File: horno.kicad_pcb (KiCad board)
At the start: 2 copper layers, 96.2 x 116 mm, 25 parts, among them T1 25, U1 AD596AHZ, U2 STM32F103C8Tx, U3 LM78M05_TO220, U4 LM78M05_TO220

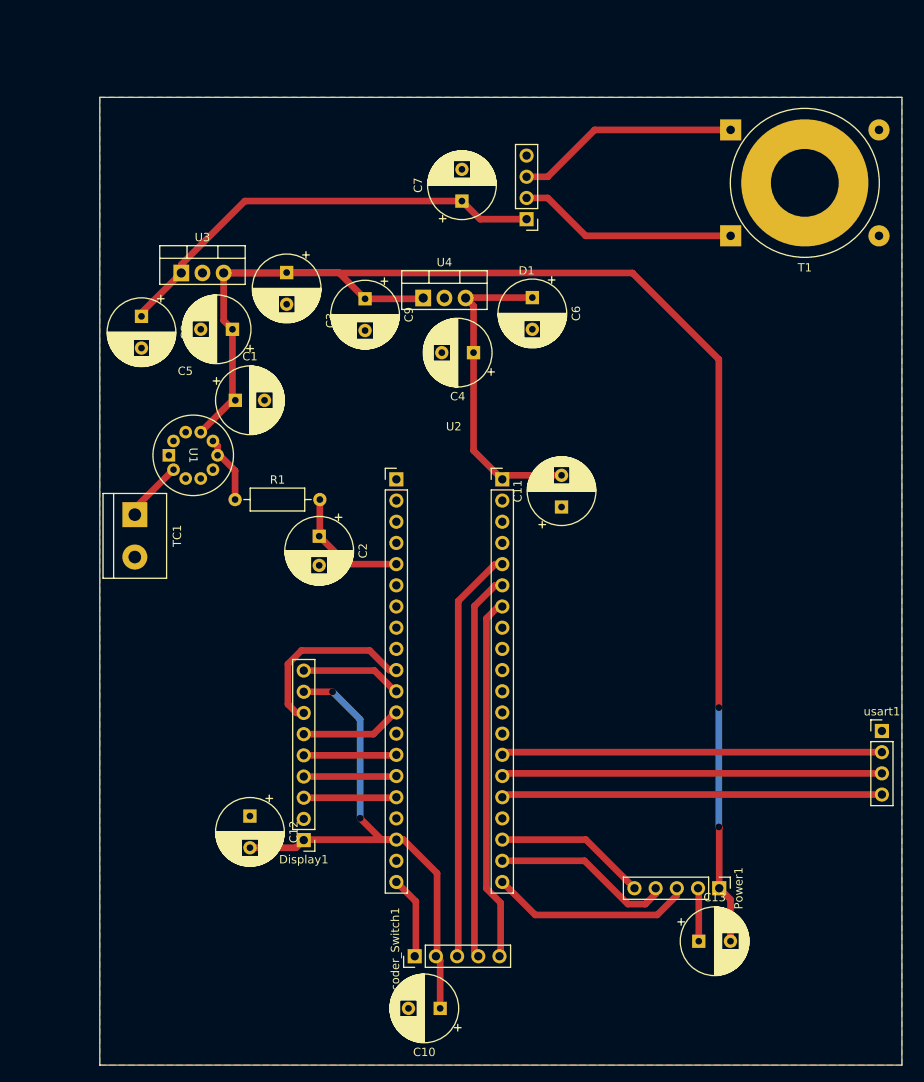
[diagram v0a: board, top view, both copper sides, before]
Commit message: com
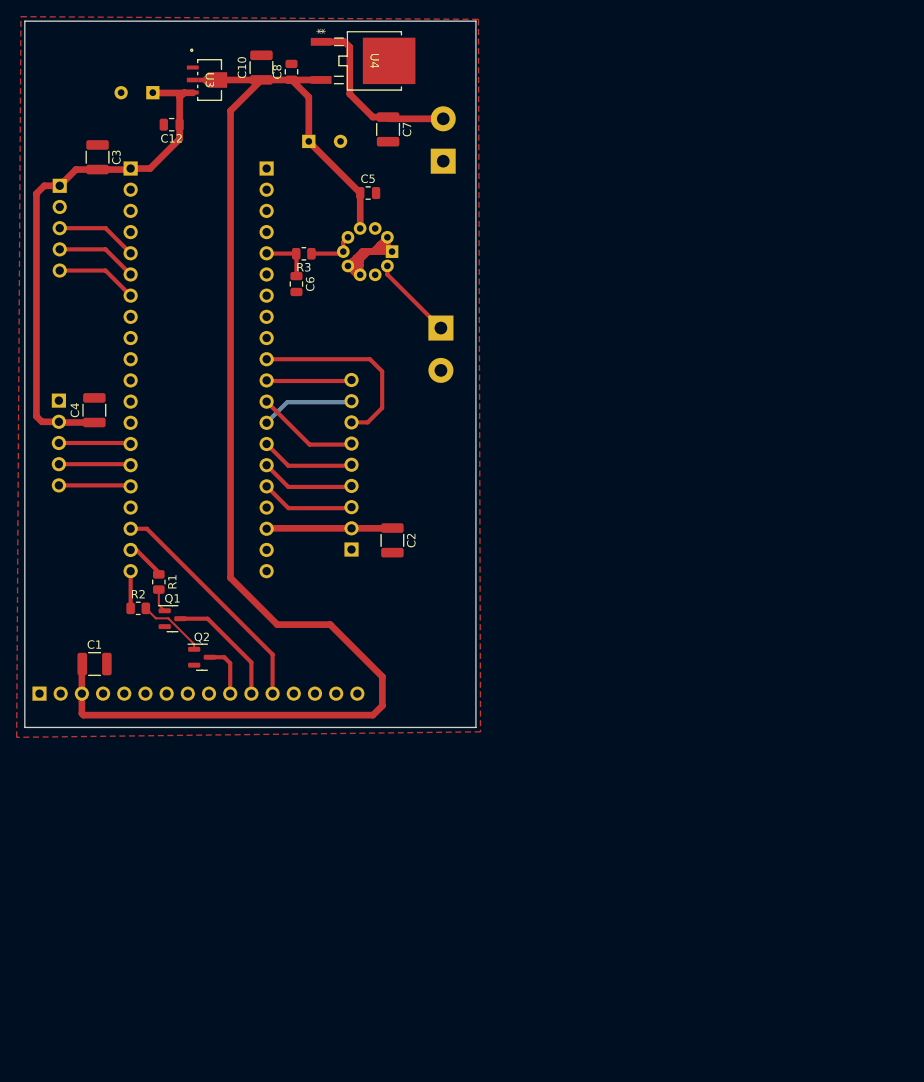
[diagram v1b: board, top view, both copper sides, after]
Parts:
- removed C13: 100n, Capacitor_THT:CP_Radial_D8.0mm_P3.80mm
- removed D1: D_Bridge_+-AA, Connector_PinHeader_2.54mm:PinHeader_1x04_P2.54mm_Vertical
- removed Power1: Conn_01x05_Pin, Connector_PinHeader_2.54mm:PinHeader_1x05_P2.54mm_Vertical
- removed T1: 25, Transformer_THT:Transformer_Toroid_Horizontal_D18.0mm
- removed usart1: Conn_01x04_Pin, Connector_PinHeader_2.54mm:PinHeader_1x04_P2.54mm_Vertical
- added PWR1: Conn_01x16_Pin, Connector_PinHeader_2.54mm:PinHeader_1x16_P2.54mm_Horizontal, B.Cu at (37.5, 178.8)
- added Q1: BC848, Package_TO_SOT_SMD:SOT-23, F.Cu at (53.5, 169.8)
- added Q2: BC848, Package_TO_SOT_SMD:SOT-23, F.Cu at (57.0, 174.5)
- added R2: 4.7k, Resistor_SMD:R_0805_2012Metric, F.Cu at (49.4, 168.6)
- added R3: 33k, Resistor_SMD:R_0805_2012Metric, F.Cu at (69.2, 126.1)
- added USART1: Conn_01x05_Pin, Connector_PinHeader_2.54mm:PinHeader_1x05_P2.54mm_Vertical, B.Cu at (39.9, 143.7)
- added Vin1: Conn_01x02, TerminalBlock:TerminalBlock_bornier-2_P5.08mm, B.Cu at (85.9, 115.0)
- C1: value 0.01u -> 100n; footprint Capacitor_THT:CP_Radial_D8.0mm_P3.50mm -> Capacitor_SMD:C_1210_3225Metric
- C10: footprint Capacitor_THT:CP_Radial_D8.0mm_P3.80mm -> Capacitor_SMD:C_1210_3225Metric
- C11, C9: value 100n -> 47u; moved to B.Cu
- C12, C8: value 100n -> 0.1u; footprint Capacitor_THT:CP_Radial_D8.0mm_P3.80mm -> Capacitor_SMD:C_0805_2012Metric
- C2: value 470n -> 100n; footprint Capacitor_THT:CP_Radial_D8.0mm_P3.50mm -> Capacitor_SMD:C_1210_3225Metric
- C3, C4: value 47u -> 100n; footprint Capacitor_THT:CP_Radial_D8.0mm_P3.80mm -> Capacitor_SMD:C_1210_3225Metric
- C5: value 0.1u -> 0.01u; footprint Capacitor_THT:CP_Radial_D8.0mm_P3.80mm -> Capacitor_SMD:C_0805_2012Metric
- C6: value 0.1u -> 470n; footprint Capacitor_THT:CP_Radial_D8.0mm_P3.80mm -> Capacitor_SMD:C_0805_2012Metric
- C7: value 470u -> 100n; footprint Capacitor_THT:CP_Radial_D8.0mm_P3.80mm -> Capacitor_SMD:C_1210_3225Metric
- Display1, Encoder_Switch1, TC1: moved to B.Cu
- R1: value 33k -> 4.7k; footprint Resistor_THT:R_Axial_DIN0207_L6.3mm_D2.5mm_P10.16mm_Horizontal -> Resistor_SMD:R_0805_2012Metric
- U1: value AD596AHZ -> STM32F103C8Tx; footprint ad596:ad596 -> blue_pill:blue_pill; moved to B.Cu
- U2: value STM32F103C8Tx -> AD596AHZ; footprint blue_pill:blue_pill -> ad596:ad596; moved to B.Cu
- U3: value LM78M05_TO220 -> MCP1700T-3302E/MB; footprint Package_TO_SOT_THT:TO-220-3_Vertical -> reg33:SOT-89_3MC_MCH
- U4: value LM78M05_TO220 -> L78M05CDT-TR; footprint Package_TO_SOT_THT:TO-220-3_Vertical -> reg5:DPAK_STM
- moved C10 114.8 mm to (64.1, 103.8), turned to 90 degrees
- moved Encoder_Switch1 101.7 mm to (40.0, 118.0), turned to 180 degrees
- moved C12 83.4 mm to (53.4, 110.6), turned to 180 degrees
- moved C11 53.3 mm to (69.8, 112.6), turned to 0 degrees
- moved C4 46.0 mm to (44.1, 144.8), turned to 90 degrees
- moved TC1 43.0 mm to (85.6, 135.0)
- moved U1 40.5 mm to (57.9, 110.0), turned to 180 degrees
- moved C1 35.8 mm to (44.1, 175.3)
- moved C9 35.5 mm to (51.1, 106.8), turned to 180 degrees
- moved Display1 35.3 mm to (74.9, 161.6), turned to 0 degrees
- moved C8 34.4 mm to (67.7, 104.3), turned to 90 degrees
- moved U4 29.0 mm to (77.7, 103.0), turned to -90 degrees
- moved C6 28.3 mm to (68.3, 129.7)
- moved C3 26.6 mm to (44.5, 114.5)
- moved U3 23.4 mm to (57.9, 105.3), turned to -90 degrees
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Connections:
- C10 pad 1: 3.3V -> 5V
- C11 pad 1: 0 -> 5V
- C11 pad 2: 3.3V -> 0
- C12 pad 1: 0 -> 3.3V
- C12 pad 2: 3.3V -> 0
- C2 pad 1: T -> 3.3V
- C3 pad 1: 5V -> 0
- C3 pad 2: 0 -> 3.3V
- C6 pad 1: 3.3V -> T
- C7 pad 1: Net-(D1-+) -> Net-(U4-INPUT)
- C8 pad 1: Net-(D1-+) -> 5V
- C9 pad 1: 5V -> 3.3V
- Display1 pad 1: 3.3V -> 0
- Display1 pad 2: 0 -> 3.3V
- Display1 pad 3: Net-(Display1-Pin_3) -> LCD_CS
- Display1 pad 4: Net-(Display1-Pin_4) -> LCD_RST
- Display1 pad 5: Net-(Display1-Pin_5) -> LCD_DC
- Display1 pad 6: Net-(Display1-Pin_6) -> LCD_MOSI
- Display1 pad 7: Net-(Display1-Pin_7) -> LCD_CLK
- Display1 pad 8: 3.3V -> LCD_LED
- Display1 pad 9: Net-(Display1-Pin_9) -> LCD_MISO
- Encoder_Switch1 pad 1: 0 -> 3.3V
- Encoder_Switch1 pad 2: 3.3V -> 0
- Encoder_Switch1 pad 3: Net-(Encoder_Switch1-Pin_3) -> IN_OK
- Encoder_Switch1 pad 4: Net-(Encoder_Switch1-Pin_4) -> IN_CH2
- Encoder_Switch1 pad 5: Net-(Encoder_Switch1-Pin_5) -> IN_CH1
- R1 pad 1: Net-(U1-FB) -> Net-(U1-PB13)
- R1 pad 2: T -> Net-(Q1-B)
- U1 pad 1: 0 -> unconnected-(U1-VBAT-Pad1)
- U1 pad 10: 0 -> T
- U1 pad 2: Net-(TC1-+) -> unconnected-(U1-PC13-Pad2)
- U1 pad 4: 0 -> unconnected-(U1-PC15-Pad4)
- U1 pad 7: Net-(U1-FB) -> unconnected-(U1-NRST-Pad7)
- U2 pad 1: unconnected-(U2-VBAT-Pad1) -> 0
- U2 pad 10: T -> 0
- U2 pad 2: unconnected-(U2-PC13-Pad2) -> Net-(TC1-+)
- U2 pad 4: unconnected-(U2-PC15-Pad4) -> 0
- U2 pad 7: unconnected-(U2-NRST-Pad7) -> Net-(U2-FB)
- U3 pad 1: Net-(D1-+) -> 0
- U3 pad 2: 0 -> 5V
- U3 pad 3: 5V -> 3.3V
- U4 pad 1: 5V -> Net-(U4-INPUT)
- U4 pad 2: 0 -> 5V
- U4 pad 3: 3.3V -> 0
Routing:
- net Net-(D1-+): track 53.6 -> 0.00 mm
- net Net-(Encoder_Switch1-Pin_3): track 49.7 -> 0.00 mm
- net Net-(Encoder_Switch1-Pin_4): track 46.5 -> 0.00 mm
- net Net-(U2-PA8): track 45.6 -> 0.00 mm
- net Net-(U2-PA9): track 45.6 -> 0.00 mm
- net Net-(U2-PA10): track 45.6 -> 0.00 mm
- net Net-(Encoder_Switch1-Pin_5): track 43.8 -> 0.00 mm
- net PWR_ZC: track 0.00 -> 28.1 mm
- net Net-(T1-SB): track 26.8 -> 0.00 mm
- net Net-(T1-SA): track 26.3 -> 0.00 mm
- net 3.3V: track 105.4 -> 79.2 mm, vias 2 -> 0
- net Net-(Power1-Pin_3): track 24.4 -> 0.00 mm
- net LCD_CLK: track 0.00 -> 23.2 mm
- net Net-(U4-INPUT): track 0.00 -> 21.9 mm
- net Net-(Display1-Pin_7): track 21.8 -> 0.00 mm
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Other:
- board size 96.2 x 116 mm -> 54.1 x 84.7 mm
